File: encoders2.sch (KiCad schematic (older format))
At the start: 45 parts, among them U7 74HCT595, U9 74HC165

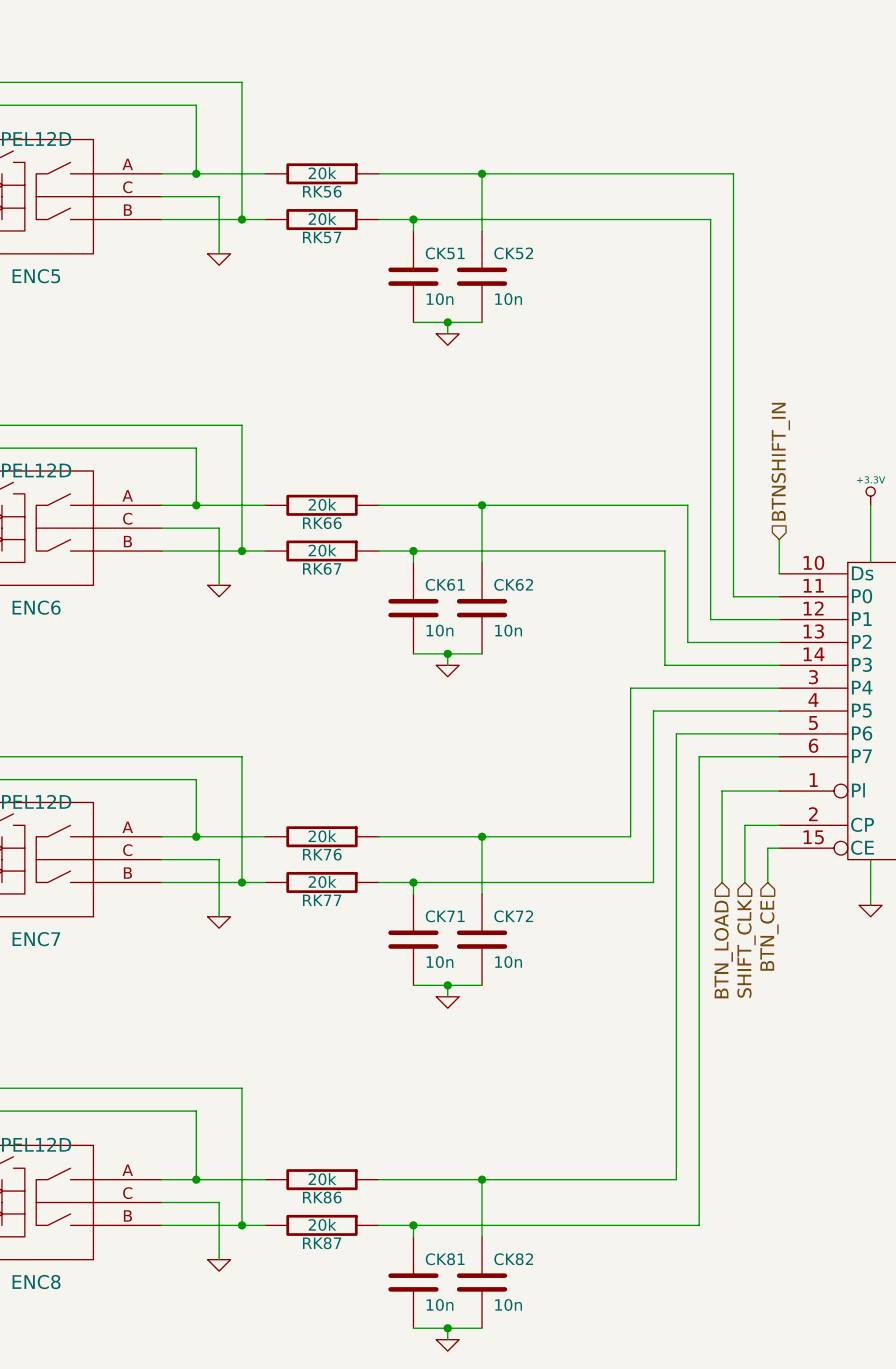
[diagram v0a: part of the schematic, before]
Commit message: Routing.
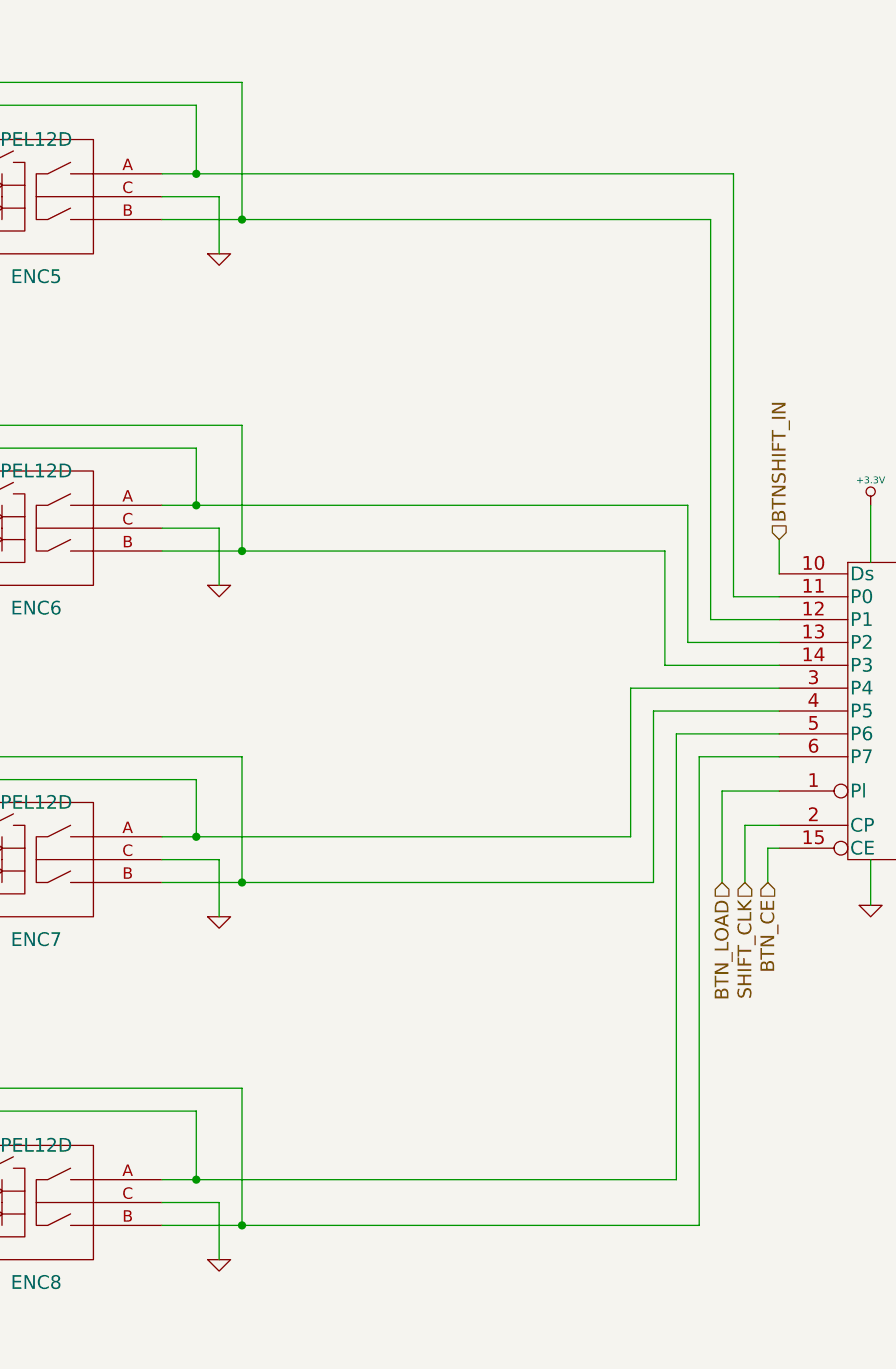
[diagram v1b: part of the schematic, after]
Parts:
- removed CK51, CK52, CK61, CK62, CK71, CK72, CK81, CK82: 10n, symbol C
- removed RK56, RK57, RK66, RK67, RK76, RK77, RK86, RK87: 20k, symbol R
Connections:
- wire segments 173 -> 149
